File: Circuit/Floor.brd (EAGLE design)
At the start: 27 parts, among them U1 AMS1117-3.3, X2 ESP-12

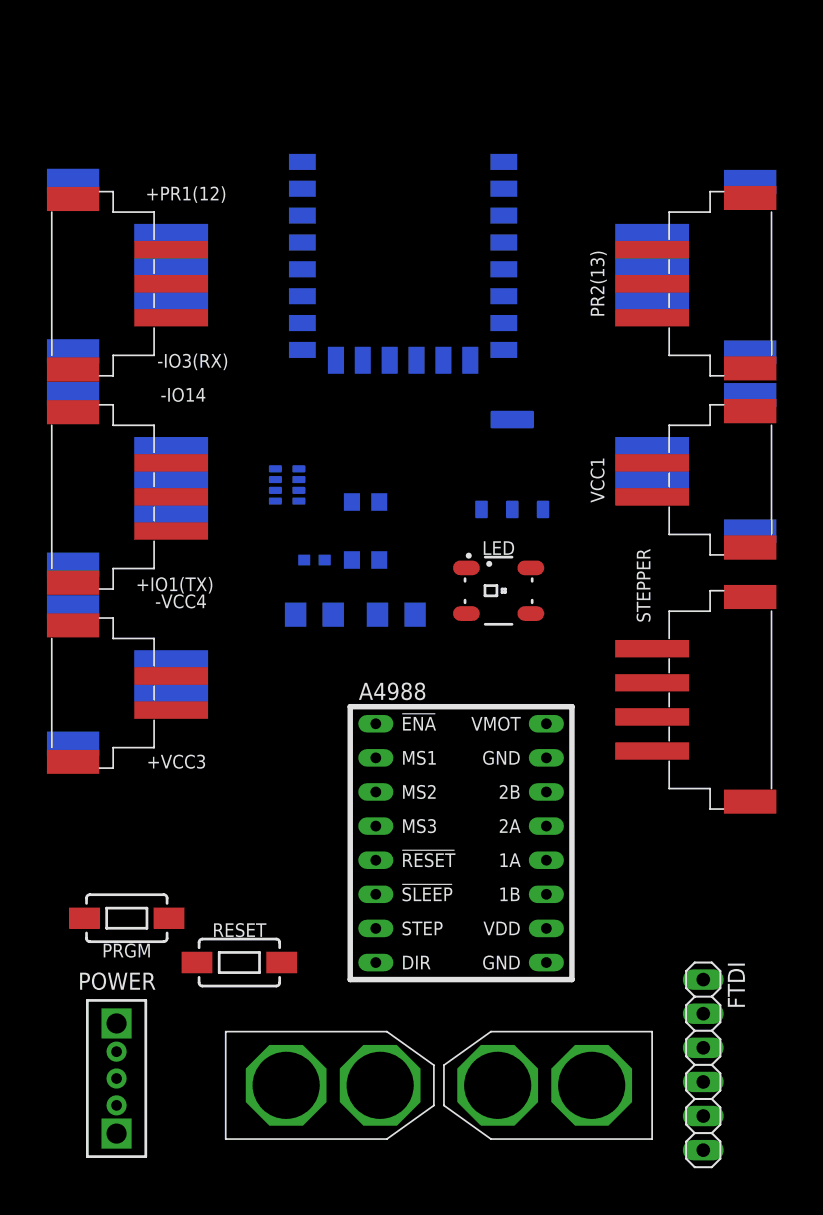
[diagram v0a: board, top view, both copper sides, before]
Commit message: floor pcb, led library, espnow wip
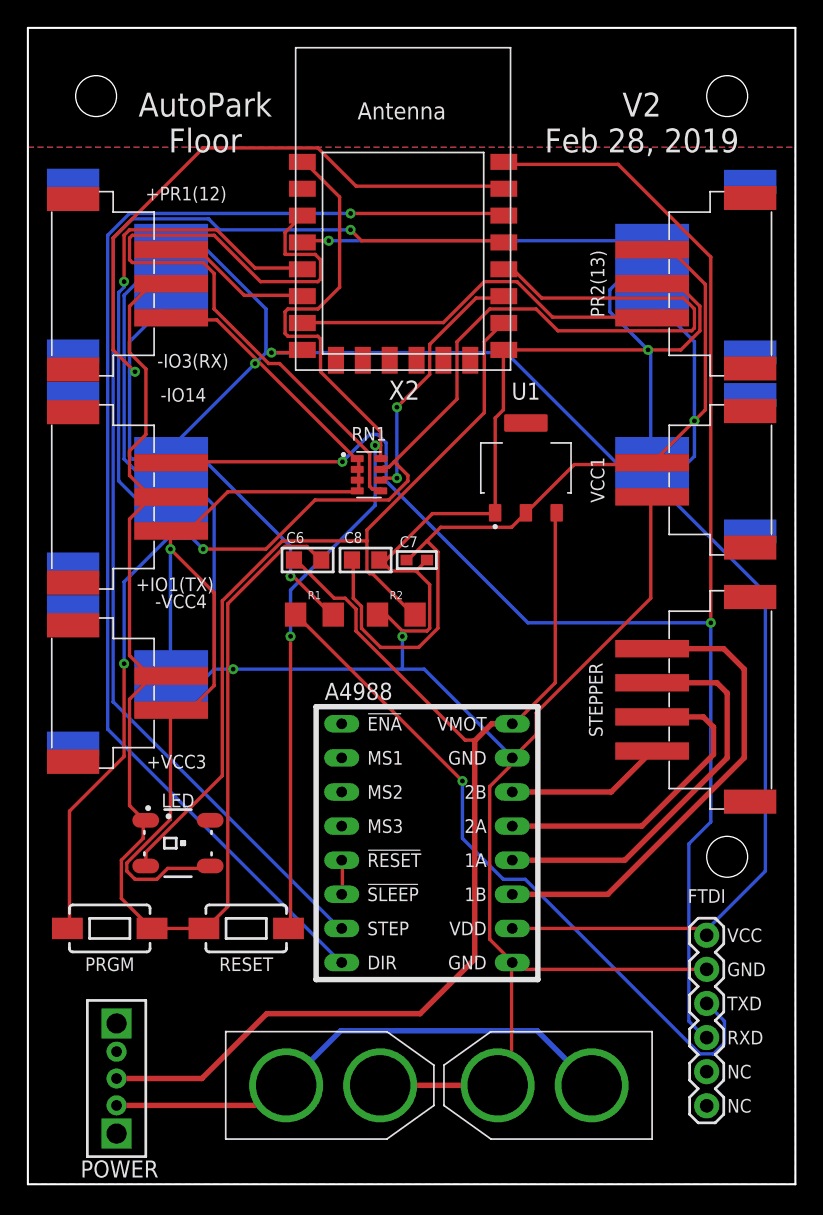
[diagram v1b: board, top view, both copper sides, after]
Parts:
- removed FTDI: (no value), pinhead:1X06
- added U$11: FTDI, AutoPark:1X06
- moved LED 30.4 mm to (9.91, 26.7)
- moved C7 7.62 mm to (27.7, 47.8), flipped to the top
- moved RN1 6.14 mm to (24.1, 54.1), flipped to the top
- moved C6 6.11 mm to (19.6, 47.8), flipped to the top
- moved RESET 2.59 mm to (15.0, 20.3)
- moved A4988 2.54 mm to (29.7, 27.9)
- moved PRGM 1.48 mm to (4.83, 20.3)
- moved U1 1.05 mm to (35.8, 54.6), flipped to the top
- flipped C8 to the top
- turned POWER to 0 degrees
- flipped R1 to the top
- flipped R2 to the top
- flipped X2 to the top
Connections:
- net 3.3V: now also U$11.VCC; no longer FTDI.1
- net GND: now also U$11.GND; no longer FTDI.2
- net TXD: now also U$11.RXD; no longer FTDI.4
- net USB_RX: now also U$11.TXD; no longer FTDI.3
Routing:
- net GND: track 0.00 -> 317.1 mm, vias 0 -> 3
- net 3.3V: track 0.00 -> 271.5 mm, vias 0 -> 4
- net TXD: track 0.00 -> 126.3 mm, vias 0 -> 2
- net GPIO0: track 0.00 -> 102.8 mm, vias 0 -> 2
- net GPIO5/SCL: track 0.00 -> 91.7 mm, vias 0 -> 1
- net GPIO4/SDA: track 0.00 -> 89.0 mm, vias 0 -> 1
- net VBAT: track 0.00 -> 87.1 mm
- net RXD: track 0.00 -> 78.5 mm, vias 0 -> 2
- net RESET: track 0.00 -> 69.7 mm, vias 0 -> 2
- net GPIO15: track 0.00 -> 62.4 mm
- net CH_PD: track 0.00 -> 54.0 mm
- net USB_RX: track 0.00 -> 51.8 mm, vias 0 -> 1
- net VIN: track 0.00 -> 39.4 mm
- net GPIO14/SCK: track 0.00 -> 38.1 mm, vias 0 -> 1
- net 1B: track 0.00 -> 35.6 mm
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- added copper zone on layer 1, net GND
- added copper zone on layer 16, net GND
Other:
- board outline added: 57.2 x 86.1 mm
- board text added: "AutoPark Floor"
- board text added: "V2 Feb 28, 2019"
